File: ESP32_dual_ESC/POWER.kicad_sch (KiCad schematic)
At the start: 30 parts, among them J1 A, J4 Conn_01x02, U12 INA219AxD, U13 MCP6002-xSN, U5 TPS5430DDA

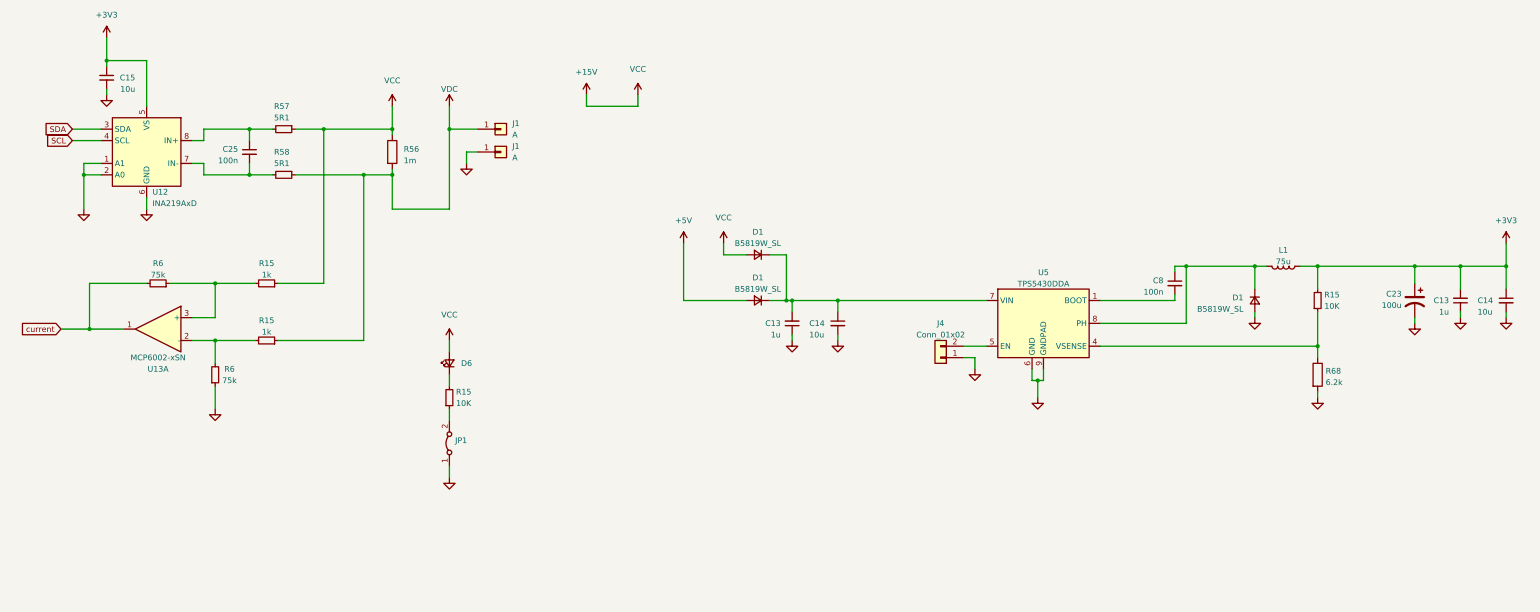
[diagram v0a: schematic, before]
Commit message: g
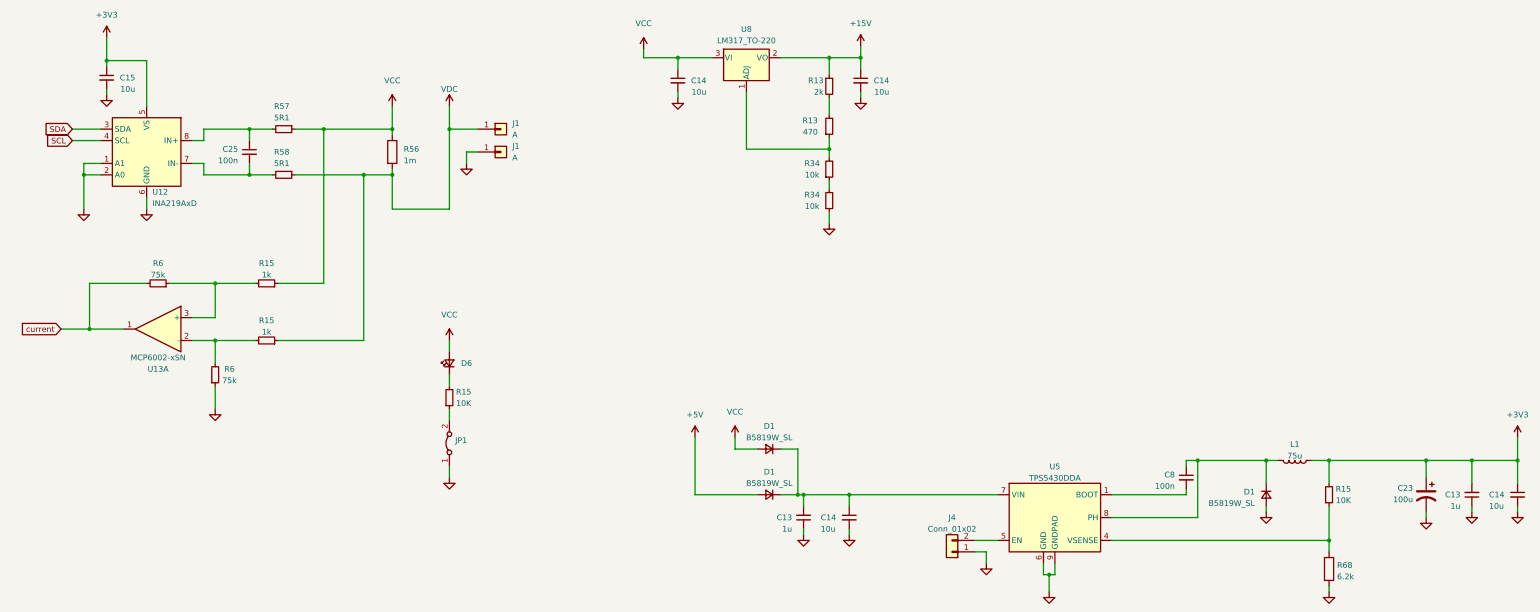
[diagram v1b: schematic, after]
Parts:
- added C14 (x2): 10u, Capacitor_SMD:C_0603_1608Metric, symbol Device:C_Small
- added R13: 2k, Resistor_SMD:R_0402_1005Metric, symbol Device:R_Small
- added R13: 470, Resistor_SMD:R_0402_1005Metric, symbol Device:R_Small
- added R34 (x2): 10k, Resistor_SMD:R_0603_1608Metric, symbol Device:R_Small
- added U8: LM317_TO-220, Package_TO_SOT_THT:TO-220-3_Vertical, symbol Regulator_Linear:LM317_TO-220
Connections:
- net +15V: now also C14.1, R13.1, U8.2 (VO); no longer D1.2 (A), D6.2 (A), R15.1, R56.1, R57.1
- net GND: now also C14.2, C14.2, R34.1
- new net: R34.1, R34.2
- new net: R13.2, R13.2
- new net: R13.1, R34.2, U8.1 (ADJ)
- new net VCC: C14.1, D1.2 (A), D6.2 (A), R15.1, R56.1, R57.1, U8.3 (VI)
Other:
- moved on the sheet: C13, C14, C23, C8, D1, J4, L1, R15, R68, U5
